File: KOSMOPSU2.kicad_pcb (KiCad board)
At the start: 2 copper layers, 153.7 x 73.9 mm, 31 parts, among them J1 Conn_01x03_Male, J2 Conn_02x05_Odd_Even, J3 Conn_01x03_Male, T1 Myrra 44440 Transformer 240V, U1 L7812, U2 L7912

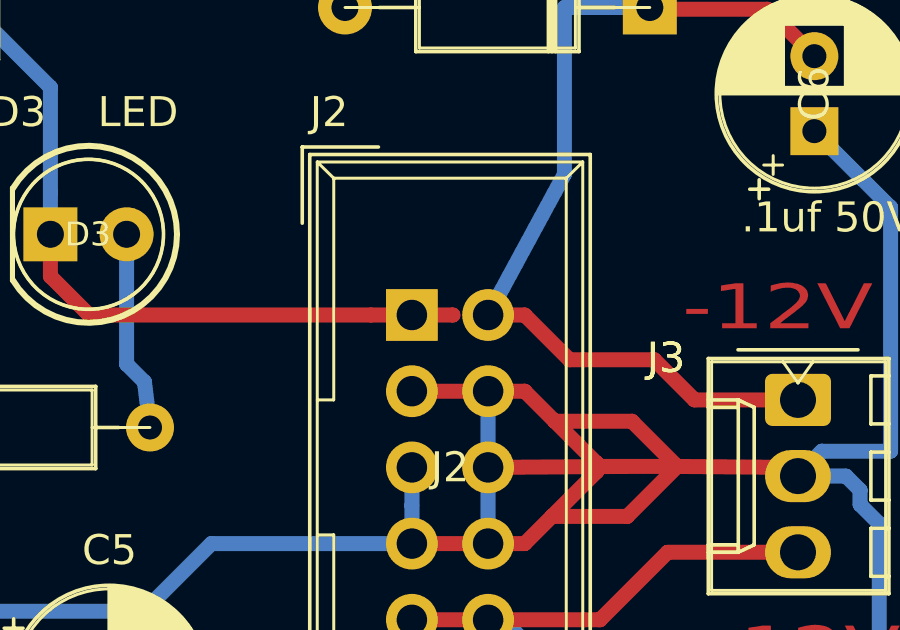
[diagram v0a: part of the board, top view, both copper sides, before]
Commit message: -12V header Fix
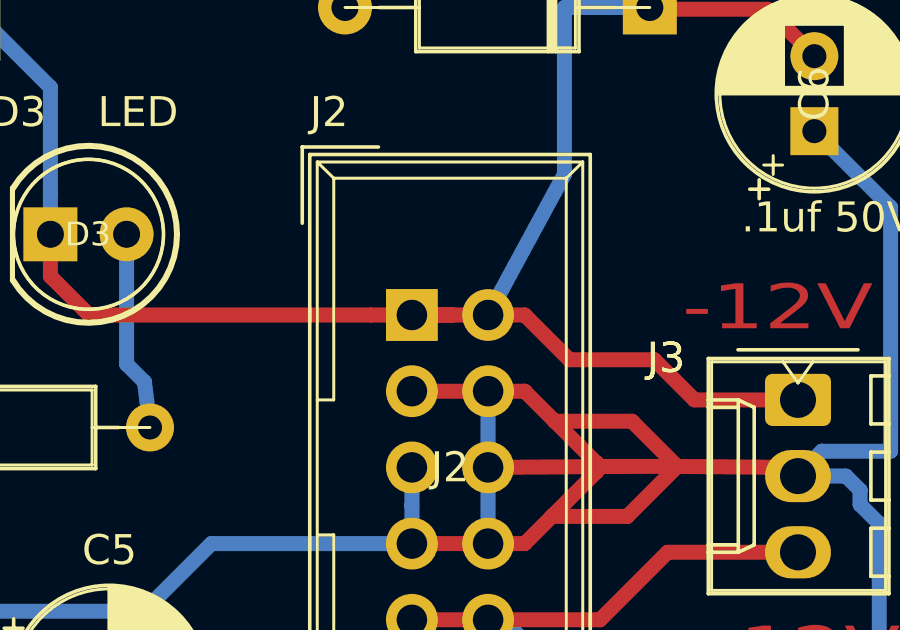
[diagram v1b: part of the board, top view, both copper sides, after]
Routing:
- net -12V: track 58.1 -> 60.6 mm
